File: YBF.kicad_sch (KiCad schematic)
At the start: 17 parts, among them J1 Chain_LED_out, J2 Chain_LED_return, SW1 1825910-6, SW2 1825910-6

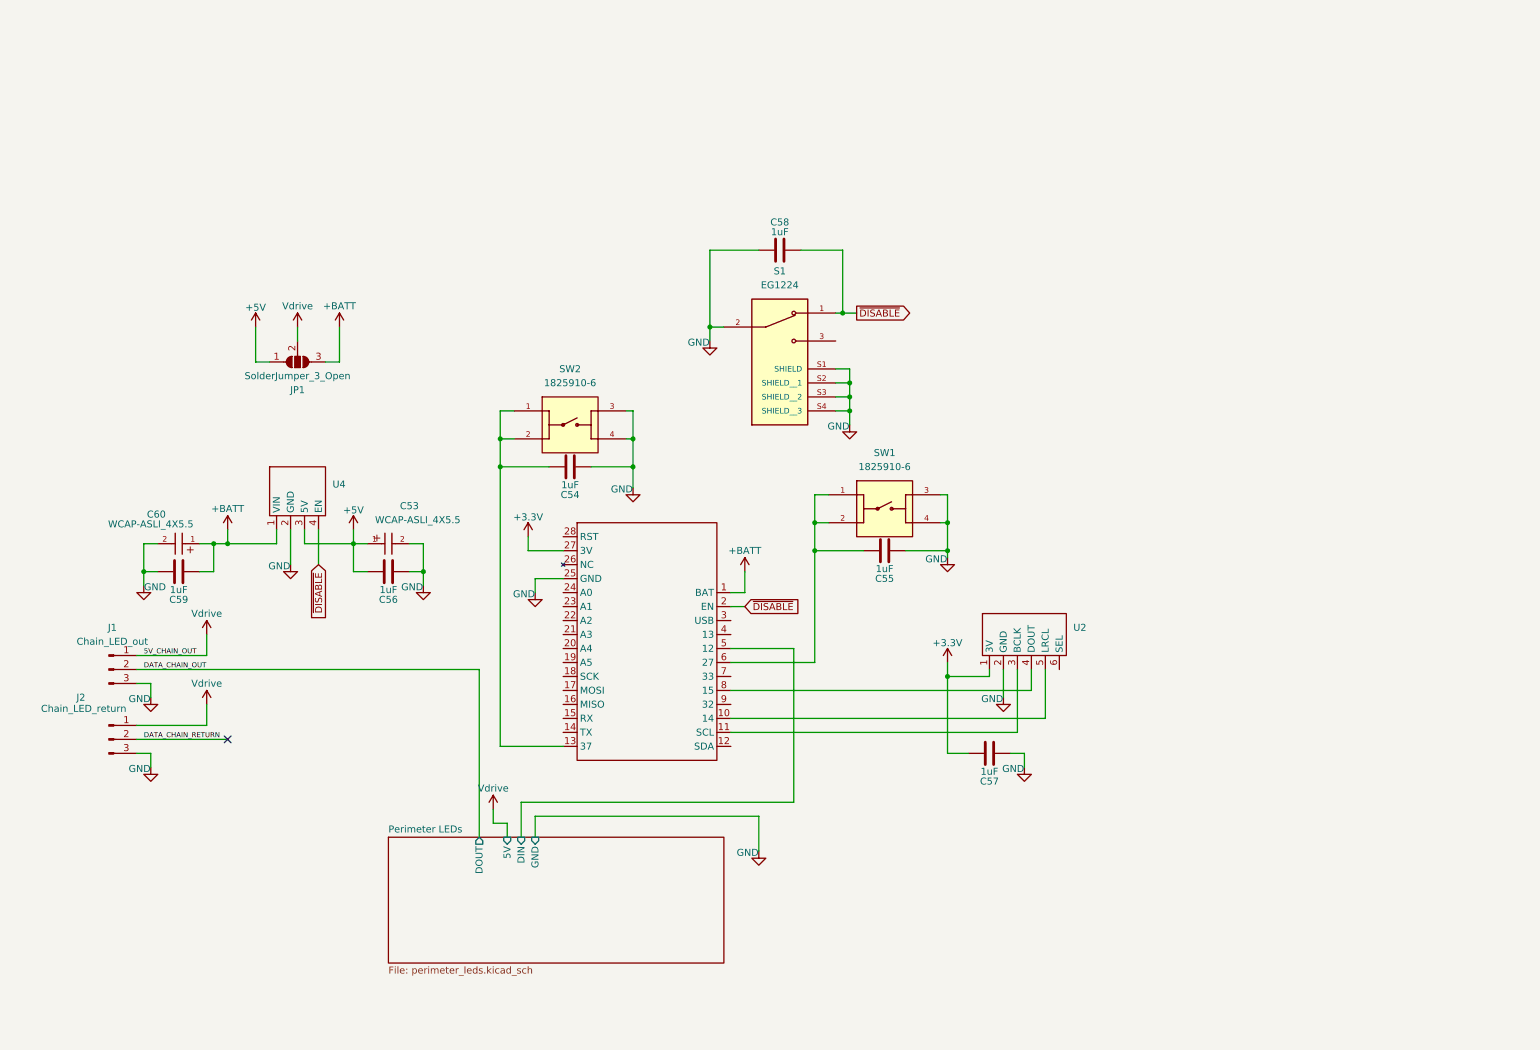
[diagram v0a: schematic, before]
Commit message: Hieracrchical PCB
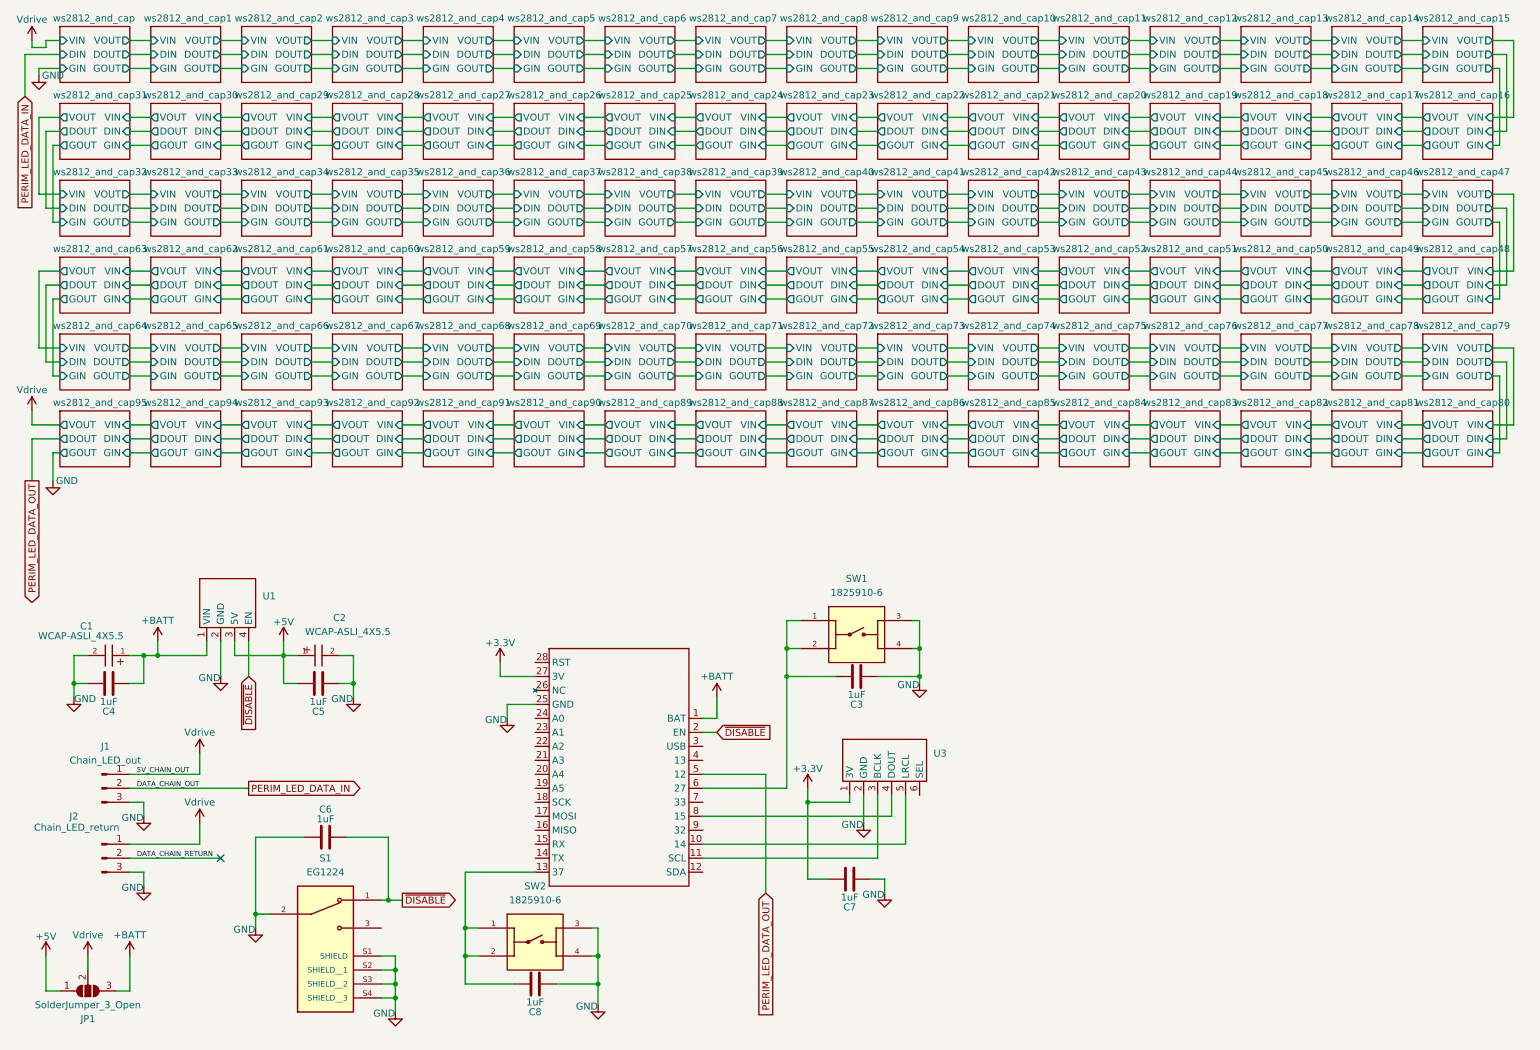
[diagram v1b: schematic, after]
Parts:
- renumbered C60 to C1, C53 to C2, C55 to C3, C59 to C4, C56 to C5, C58 to C6, C57 to C7, C54 to C8, U4 to U1, U1 to U2, U2 to U3
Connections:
- net DATA_CHAIN_OUT renamed PERIM_LED_DATA_IN
- net Perimeter LEDs/DIN renamed PERIM_LED_DATA_OUT
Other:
- removed sheet Perimeter LEDs
- added sheet ws2812_and_cap (ws2812_and_cap.kicad_sch)
- added sheet ws2812_and_cap1 (ws2812_and_cap.kicad_sch)
- added sheet ws2812_and_cap10 (ws2812_and_cap.kicad_sch)
- added sheet ws2812_and_cap11 (ws2812_and_cap.kicad_sch)
- added sheet ws2812_and_cap12 (ws2812_and_cap.kicad_sch)
- added sheet ws2812_and_cap13 (ws2812_and_cap.kicad_sch)
- added sheet ws2812_and_cap14 (ws2812_and_cap.kicad_sch)
- added sheet ws2812_and_cap15 (ws2812_and_cap.kicad_sch)
- added sheet ws2812_and_cap16 (ws2812_and_cap.kicad_sch)
- added sheet ws2812_and_cap17 (ws2812_and_cap.kicad_sch)
- added sheet ws2812_and_cap18 (ws2812_and_cap.kicad_sch)
- added sheet ws2812_and_cap19 (ws2812_and_cap.kicad_sch)
- added sheet ws2812_and_cap2 (ws2812_and_cap.kicad_sch)
- added sheet ws2812_and_cap20 (ws2812_and_cap.kicad_sch)
- added sheet ws2812_and_cap21 (ws2812_and_cap.kicad_sch)
- added sheet ws2812_and_cap22 (ws2812_and_cap.kicad_sch)
- added sheet ws2812_and_cap23 (ws2812_and_cap.kicad_sch)
- added sheet ws2812_and_cap24 (ws2812_and_cap.kicad_sch)
- added sheet ws2812_and_cap25 (ws2812_and_cap.kicad_sch)
- added sheet ws2812_and_cap26 (ws2812_and_cap.kicad_sch)
- added sheet ws2812_and_cap27 (ws2812_and_cap.kicad_sch)
- added sheet ws2812_and_cap28 (ws2812_and_cap.kicad_sch)
- added sheet ws2812_and_cap29 (ws2812_and_cap.kicad_sch)
- added sheet ws2812_and_cap3 (ws2812_and_cap.kicad_sch)
- added sheet ws2812_and_cap30 (ws2812_and_cap.kicad_sch)
- added sheet ws2812_and_cap31 (ws2812_and_cap.kicad_sch)
- added sheet ws2812_and_cap32 (ws2812_and_cap.kicad_sch)
- added sheet ws2812_and_cap33 (ws2812_and_cap.kicad_sch)
- added sheet ws2812_and_cap34 (ws2812_and_cap.kicad_sch)
- added sheet ws2812_and_cap35 (ws2812_and_cap.kicad_sch)
- added sheet ws2812_and_cap36 (ws2812_and_cap.kicad_sch)
- added sheet ws2812_and_cap37 (ws2812_and_cap.kicad_sch)
- added sheet ws2812_and_cap38 (ws2812_and_cap.kicad_sch)
- added sheet ws2812_and_cap39 (ws2812_and_cap.kicad_sch)
- added sheet ws2812_and_cap4 (ws2812_and_cap.kicad_sch)
- added sheet ws2812_and_cap40 (ws2812_and_cap.kicad_sch)
- added sheet ws2812_and_cap41 (ws2812_and_cap.kicad_sch)
- added sheet ws2812_and_cap42 (ws2812_and_cap.kicad_sch)
- added sheet ws2812_and_cap43 (ws2812_and_cap.kicad_sch)
- added sheet ws2812_and_cap44 (ws2812_and_cap.kicad_sch)
- added sheet ws2812_and_cap45 (ws2812_and_cap.kicad_sch)
- added sheet ws2812_and_cap46 (ws2812_and_cap.kicad_sch)
- added sheet ws2812_and_cap47 (ws2812_and_cap.kicad_sch)
- added sheet ws2812_and_cap48 (ws2812_and_cap.kicad_sch)
- added sheet ws2812_and_cap49 (ws2812_and_cap.kicad_sch)
- added sheet ws2812_and_cap5 (ws2812_and_cap.kicad_sch)
- added sheet ws2812_and_cap50 (ws2812_and_cap.kicad_sch)
- added sheet ws2812_and_cap51 (ws2812_and_cap.kicad_sch)
- added sheet ws2812_and_cap52 (ws2812_and_cap.kicad_sch)
- added sheet ws2812_and_cap53 (ws2812_and_cap.kicad_sch)
- added sheet ws2812_and_cap54 (ws2812_and_cap.kicad_sch)
- added sheet ws2812_and_cap55 (ws2812_and_cap.kicad_sch)
- added sheet ws2812_and_cap56 (ws2812_and_cap.kicad_sch)
- added sheet ws2812_and_cap57 (ws2812_and_cap.kicad_sch)
- added sheet ws2812_and_cap58 (ws2812_and_cap.kicad_sch)
- added sheet ws2812_and_cap59 (ws2812_and_cap.kicad_sch)
- added sheet ws2812_and_cap6 (ws2812_and_cap.kicad_sch)
- added sheet ws2812_and_cap60 (ws2812_and_cap.kicad_sch)
- added sheet ws2812_and_cap61 (ws2812_and_cap.kicad_sch)
- added sheet ws2812_and_cap62 (ws2812_and_cap.kicad_sch)
- added sheet ws2812_and_cap63 (ws2812_and_cap.kicad_sch)
- added sheet ws2812_and_cap64 (ws2812_and_cap.kicad_sch)
- added sheet ws2812_and_cap65 (ws2812_and_cap.kicad_sch)
- added sheet ws2812_and_cap66 (ws2812_and_cap.kicad_sch)
- added sheet ws2812_and_cap67 (ws2812_and_cap.kicad_sch)
- added sheet ws2812_and_cap68 (ws2812_and_cap.kicad_sch)
- added sheet ws2812_and_cap69 (ws2812_and_cap.kicad_sch)
- added sheet ws2812_and_cap7 (ws2812_and_cap.kicad_sch)
- added sheet ws2812_and_cap70 (ws2812_and_cap.kicad_sch)
- added sheet ws2812_and_cap71 (ws2812_and_cap.kicad_sch)
- added sheet ws2812_and_cap72 (ws2812_and_cap.kicad_sch)
- added sheet ws2812_and_cap73 (ws2812_and_cap.kicad_sch)
- added sheet ws2812_and_cap74 (ws2812_and_cap.kicad_sch)
- added sheet ws2812_and_cap75 (ws2812_and_cap.kicad_sch)
- added sheet ws2812_and_cap76 (ws2812_and_cap.kicad_sch)
- added sheet ws2812_and_cap77 (ws2812_and_cap.kicad_sch)
- added sheet ws2812_and_cap78 (ws2812_and_cap.kicad_sch)
- added sheet ws2812_and_cap79 (ws2812_and_cap.kicad_sch)
- added sheet ws2812_and_cap8 (ws2812_and_cap.kicad_sch)
- added sheet ws2812_and_cap80 (ws2812_and_cap.kicad_sch)
- added sheet ws2812_and_cap81 (ws2812_and_cap.kicad_sch)
- added sheet ws2812_and_cap82 (ws2812_and_cap.kicad_sch)
- added sheet ws2812_and_cap83 (ws2812_and_cap.kicad_sch)
- added sheet ws2812_and_cap84 (ws2812_and_cap.kicad_sch)
- added sheet ws2812_and_cap85 (ws2812_and_cap.kicad_sch)
- added sheet ws2812_and_cap86 (ws2812_and_cap.kicad_sch)
- added sheet ws2812_and_cap87 (ws2812_and_cap.kicad_sch)
- added sheet ws2812_and_cap88 (ws2812_and_cap.kicad_sch)
- added sheet ws2812_and_cap89 (ws2812_and_cap.kicad_sch)
- added sheet ws2812_and_cap9 (ws2812_and_cap.kicad_sch)
- added sheet ws2812_and_cap90 (ws2812_and_cap.kicad_sch)
- added sheet ws2812_and_cap91 (ws2812_and_cap.kicad_sch)
- added sheet ws2812_and_cap92 (ws2812_and_cap.kicad_sch)
- added sheet ws2812_and_cap93 (ws2812_and_cap.kicad_sch)
- added sheet ws2812_and_cap94 (ws2812_and_cap.kicad_sch)
- added sheet ws2812_and_cap95 (ws2812_and_cap.kicad_sch)
- moved on the sheet: C1, C2, C3, C4, C5, C6, C7, C8, J1, J2, JP1, S1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
